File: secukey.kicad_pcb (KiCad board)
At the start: 2 copper layers, 25 x 42 mm, 44 parts, among them SW4 TS-1185-W-4P-H1.8-160, SW5 TS-1185-W-4P-H1.8-160, SW6 TS-1185-W-4P-H1.8-160, U2 RP2350A, U3 NCP1117-3.3_SOT223, U4 W25Q128JVS, U5 ABM8-272-T3_C20625731, U6 SM03B-SRSS-TB, U7 ATECC608A-MAHDA-T

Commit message: adding ref
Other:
- rule pad_to_mask_clearance: 0.05 -> 0.1
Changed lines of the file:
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@@
 	(layers
 		(0 "F.Cu" signal)
-		(2 "B.Cu" signal)
+		(2 "B.Cu" power)
 		(9 "F.Adhes" user "F.Adhesive")
 		(11 "B.Adhes" user "B.Adhesive")
@@
 		(35 "F.Fab" user)
 		(33 "B.Fab" user)
-		(39 "User.1" user)
-		(41 "User.2" user)
-		(43 "User.3" user)
-		(45 "User.4" user)
 	)
 	(setup
@@
 				(type "Bottom Silk Screen")
 			)
-			(copper_finish "None")
+			(copper_finish "HAL lead-free")
 			(dielectric_constraints no)
 		)
-		(pad_to_mask_clearance 0.05)
+		(pad_to_mask_clearance 0.1)
+		(solder_mask_min_width 0.1)
 		(allow_soldermask_bridges_in_footprints no)
 		(tenting

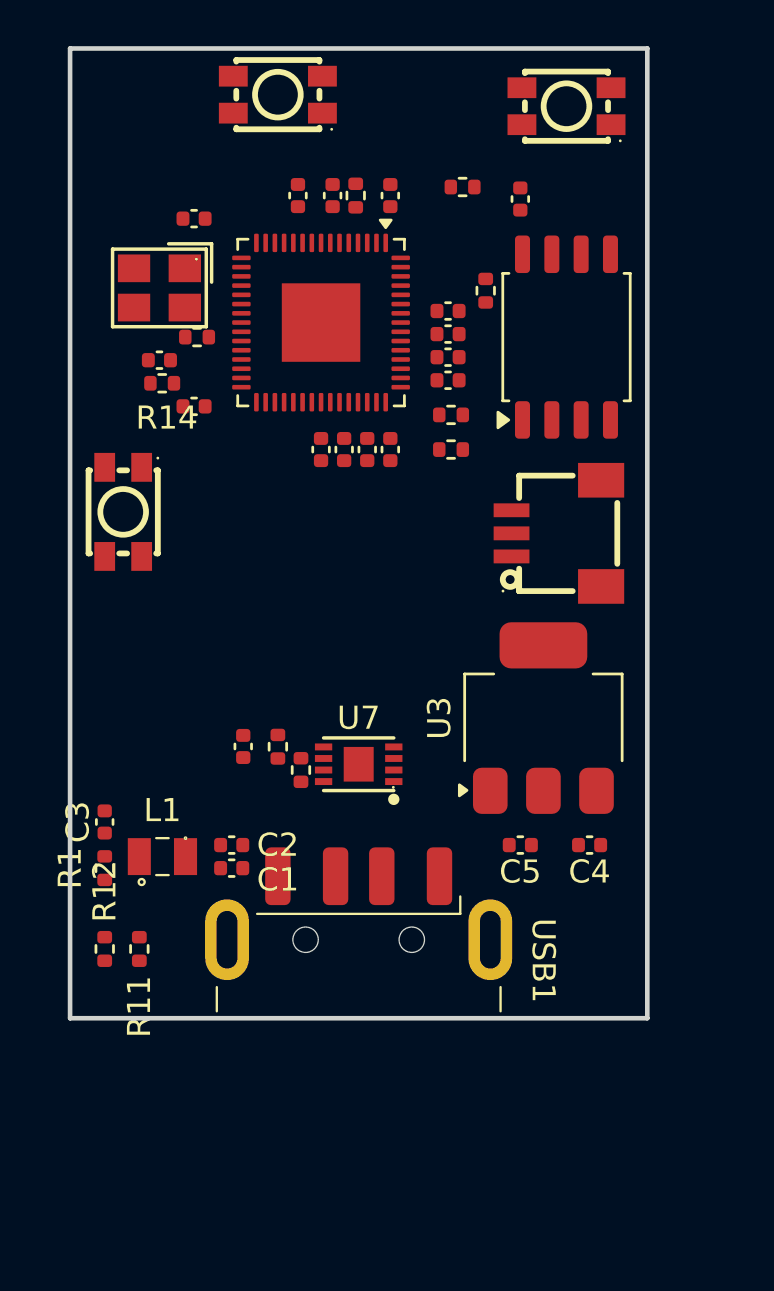
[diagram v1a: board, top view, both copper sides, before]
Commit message: adding made placement
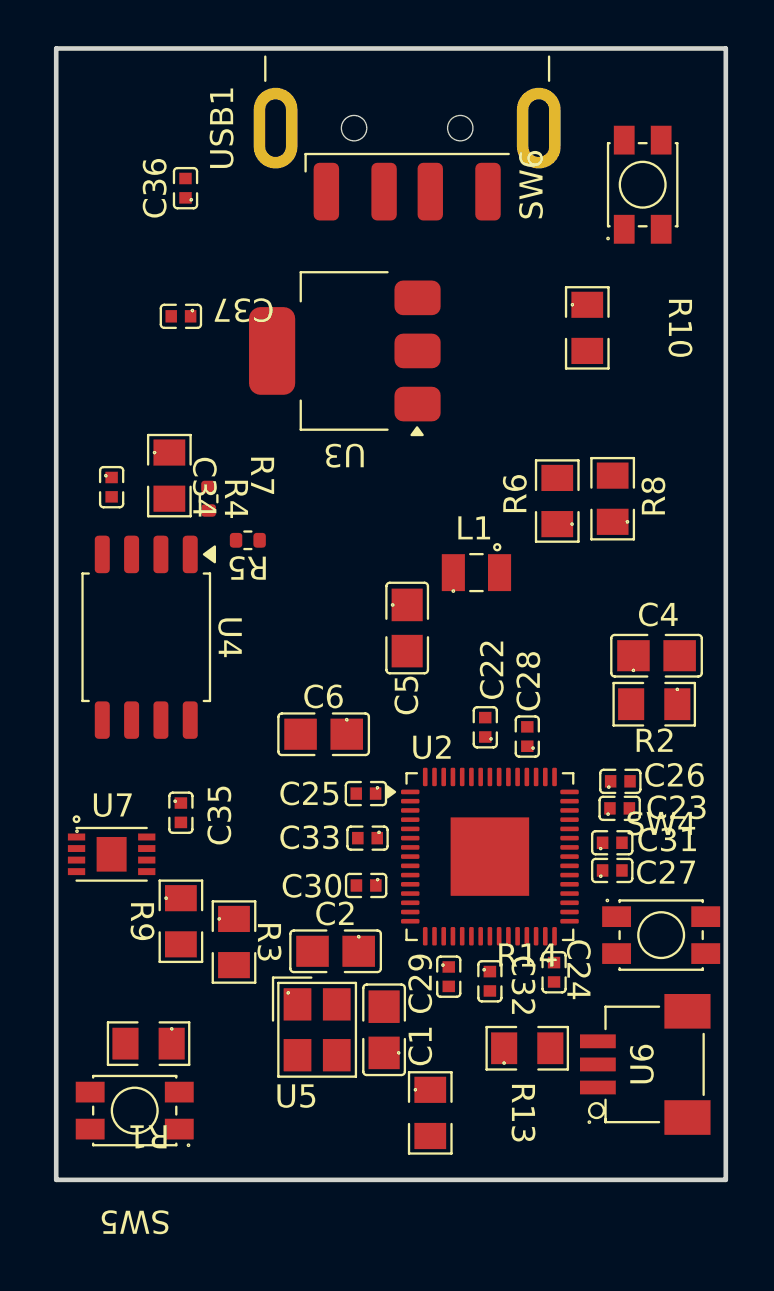
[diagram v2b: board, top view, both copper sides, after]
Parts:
- removed C10, C11, C12, C13, C14, C15, C16, C18, C7, C8, C9: 100n, Capacitor_SMD:C_0402_1005Metric
- removed C17, C3: 4.7u, Capacitor_SMD:C_0402_1005Metric
- removed C19, C20: 15p, Capacitor_SMD:C_0402_1005Metric
- removed C21: 100nF, Capacitor_SMD:C_0402_1005Metric
- removed R11, R12: 27, Resistor_SMD:R_0402_1005Metric
- added C22: CC0402KRX7R5BB104, EasyEDA:C0402, F.Cu at (163.0, 109.4)
- added C23: CC0402KRX7R5BB104, EasyEDA:C0402, F.Cu at (168.8, 112.9)
- added C24: CC0402KRX7R5BB104, EasyEDA:C0402, F.Cu at (166.0, 120.0)
- added C25: CC0402KRX7R5BB104, EasyEDA:C0402, F.Cu at (157.8, 112.3)
- added C26: CC0402KRX7R5BB104, EasyEDA:C0402, F.Cu at (168.8, 111.7)
- added C27: CC0402KRX7R5BB104, EasyEDA:C0402, F.Cu at (168.5, 115.6)
- added C28: CC0402KRX7R5BB104, EasyEDA:C0402, F.Cu at (164.8, 109.8)
- added C29: CC0402KRX7R5BB104, EasyEDA:C0402, F.Cu at (161.4, 120.2)
- added C30: CC0402KRX7R5BB104, EasyEDA:C0402, F.Cu at (157.8, 116.2)
- added C31: CC0402KRX7R5BB104, EasyEDA:C0402, F.Cu at (168.5, 114.4)
- added C32: CC0402KRX7R5BB104, EasyEDA:C0402, F.Cu at (163.2, 120.4)
- added C33: CC0402KRX7R5BB104, EasyEDA:C0402, F.Cu at (157.9, 114.2)
- added C34: CC0402KRX7R5BB104, EasyEDA:C0402, F.Cu at (146.8, 99.0)
- added C35: CC0402KRX7R5BB104, EasyEDA:C0402, F.Cu at (149.8, 113.1)
- added C36: CC0402KRX7R5BB104, EasyEDA:C0402, F.Cu at (150.0, 86.0)
- added C37: CC0402KRX7R5BB104, EasyEDA:C0402, F.Cu at (149.8, 91.6)
- added R2: 0805W8J0330T5E, EasyEDA:R0805, F.Cu at (170.3, 108.4)
- added R3: 0805W8F4701T5E, EasyEDA:R0805, F.Cu at (152.1, 118.7)
- C1, C2: value 4.7u -> FCC0805N150J500BT; footprint Capacitor_SMD:C_0402_1005Metric -> EasyEDA:C0805
- C4, C5: value 10u -> CL21A475KBQNNNE; footprint Capacitor_SMD:C_0402_1005Metric -> EasyEDA:C0805
- C6: value 100n -> CL21A475KBQNNNE; footprint Capacitor_SMD:C_0402_1005Metric -> EasyEDA:C0805
- R1: value 33Ω -> RC0805JR-0710KL; footprint Resistor_SMD:R_0402_1005Metric -> EasyEDA:R0805
- R10: value 4,7kΩ -> RC0805JR-071KL; footprint Resistor_SMD:R_0402_1005Metric -> EasyEDA:R0805
- R13: value 10kΩ -> RC0805JR-071KL; footprint Resistor_SMD:R_0402_1005Metric -> EasyEDA:R0805
- R14: value 1k -> RC0805JR-071KL; footprint Resistor_SMD:R_0402_1005Metric -> EasyEDA:R0805
- R6: value 0 -> FRC0805F27R0TS; footprint Resistor_SMD:R_0402_1005Metric -> EasyEDA:R0805
- R7: value 1k -> 0805W8F0000T5E; footprint Resistor_SMD:R_0402_1005Metric -> EasyEDA:R0805
- R8: value 1k -> FRC0805F27R0TS; footprint Resistor_SMD:R_0402_1005Metric -> EasyEDA:R0805
- R9: value 4,7kΩ -> 0805W8F4701T5E; footprint Resistor_SMD:R_0402_1005Metric -> EasyEDA:R0805
- moved USB1 49.0 mm to (159.6, 76.5), turned to 90 degrees
- moved SW5 44.4 mm to (147.8, 126.0)
- moved R13 39.9 mm to (160.6, 126.1), turned to -90 degrees
- moved R14 32.9 mm to (164.8, 123.3)
- moved U5 32.8 mm to (155.7, 122.5), turned to -90 degrees
- moved SW4 29.6 mm to (170.6, 118.4), turned to 0 degrees
- moved U2 24.3 mm to (163.2, 115.0), turned to 0 degrees
- moved U6 23.3 mm to (169.8, 124.0)
- moved R10 22.8 mm to (167.4, 92.1)
- moved U4 22.4 mm to (148.3, 105.5), turned to -90 degrees
- moved R8 19.3 mm to (168.5, 99.5), turned to 90 degrees
- moved L1 18.3 mm to (162.6, 102.7), turned to 0 degrees
- moved U3 18.1 mm to (156.9, 93.1), turned to 180 degrees
- moved R7 17.8 mm to (149.3, 98.5), turned to -90 degrees
- moved R4 15.0 mm to (151.0, 99.5)
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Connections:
- C1 pad 1: RP2350B_VREG-VIN -> Net-(C1-Pad1)
- C2 pad 1: RP2350B_VREG-FB -> RP2350B_VREG-PGND
- C2 pad 2: RP2350B_VREG-PGND -> RP2350B_XIN
- C4 pad 1: VBUS -> RP2350B_VREG-AVDD
- C5 pad 1: RP2350B_VREG-VIN -> RP2350B_VREG-FB
- R1 pad 1: RP2350B_VREG-VIN -> RP2350B_GPIO2
- R1 pad 2: RP2350B_VREG-AVDD -> RP2350B_VREG-VIN
- R10 pad 1: RP2350B_GPIO5 -> Net-(R10-Pad1)
- R10 pad 2: RP2350B_VREG-VIN -> RP2350B_QSPI_SS
- R13 pad 1: RP2350B_GPIO2 -> Net-(C1-Pad1)
- R13 pad 2: RP2350B_VREG-VIN -> RP2350B_XOUT
- R14 pad 1: Net-(R14-Pad1) -> Net-(U2-RUN)
- R14 pad 2: Net-(U2-RUN) -> Net-(R14-Pad2)
- R6 pad 1: RP2350B_QSPI_SS -> Net-(U2-USB_DP)
- R6 pad 2: Net-(U4-~{CS}) -> /USB_D-
- R7 pad 1: Net-(R7-Pad1) -> RP2350B_QSPI_SS
- R7 pad 2: RP2350B_QSPI_SS -> Net-(U4-~{CS})
- R8 pad 1: Net-(C20-Pad2) -> Net-(U2-USB_DM)
- R8 pad 2: RP2350B_XOUT -> /USB_D+
- SW4 pad 4: Net-(R14-Pad1) -> Net-(R14-Pad2)
- SW6 pad 3: Net-(R7-Pad1) -> Net-(R10-Pad1)
- U2 pad 7: unconnected-(U2-GPIO4-Pad7) -> RP2350B_GPIO4
- U2 pad 8: unconnected-(U2-GPIO5-Pad8) -> RP2350B_GPIO5
- U4 pad 2: unconnected-(U4-DO/IO_{1}-Pad2) -> RP2350B_QSPI_SD1
- U4 pad 3: unconnected-(U4-~{WP}/IO_{2}-Pad3) -> RP2350B_QSPI_SD2
- U4 pad 5: unconnected-(U4-DI/IO_{0}-Pad5) -> RP2350B_QSPI_SD0
- U4 pad 7: unconnected-(U4-~{HOLD}/~{RESET}/IO_{3}-Pad7) -> RP2350B_QSPI_SD3
- U5 pad 3: Net-(C20-Pad2) -> Net-(C1-Pad1)
- U7 pad 1: unconnected-(U7-NC-Pad1) -> RP2350B_VREG-PGND
- U7 pad 2: unconnected-(U7-NC-Pad2) -> RP2350B_VREG-PGND
- U7 pad 3: unconnected-(U7-NC-Pad3) -> RP2350B_VREG-PGND
- U7 pad 7: unconnected-(U7-NC-Pad7) -> RP2350B_VREG-PGND
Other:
- board size 25 x 42 mm -> 29 x 49 mm
